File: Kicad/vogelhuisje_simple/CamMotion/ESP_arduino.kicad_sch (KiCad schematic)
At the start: 2 parts

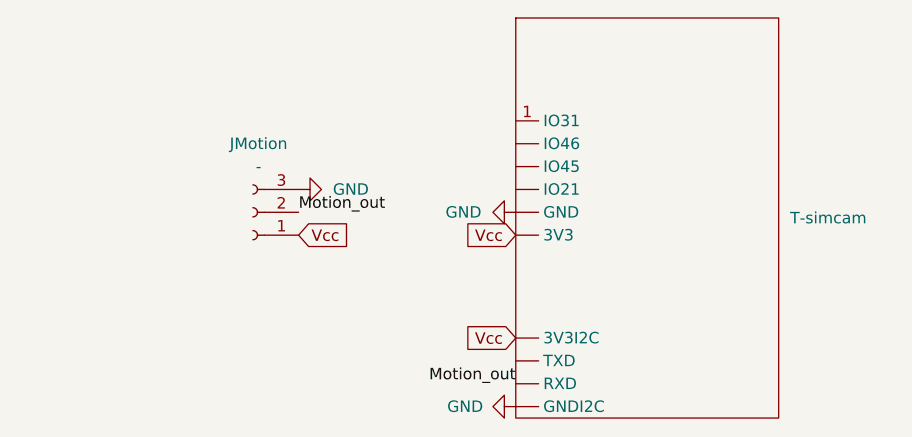
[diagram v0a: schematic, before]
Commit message: Finish pcb simplified
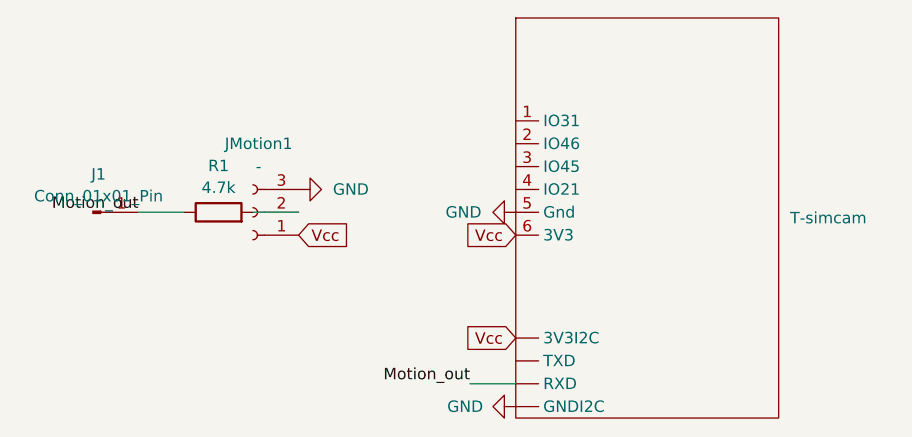
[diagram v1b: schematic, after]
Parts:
- added J1: Conn_01x01_Pin, Connector_PinHeader_2.54mm:PinHeader_1x01_P2.54mm_Vertical, symbol Connector:Conn_01x01_Pin
- added R1: 4.7k, Resistor_THT:R_Axial_DIN0204_L3.6mm_D1.6mm_P7.62mm_Horizontal, symbol Device:R
- JMotion1: renamed from JMotion; footprint (none) -> Connector_PinSocket_2.54mm:PinSocket_1x03_P2.54mm_Vertical
- U1: renamed from U?; footprint (none) -> LilyGo:TSimCam
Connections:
- net GND: now also U1.5 (Gnd)
- net Motion_out: now also J1.1 (Pin_1), R1.1; no longer JMotion1.2 (Pin_2)
- net Vcc: now also U1.6 (3V3)
- new net: JMotion1.2 (Pin_2), R1.2
